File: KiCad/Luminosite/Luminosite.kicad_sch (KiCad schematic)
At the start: 1 part, among them U4 ESP32-C3_SUPERMINI_TH

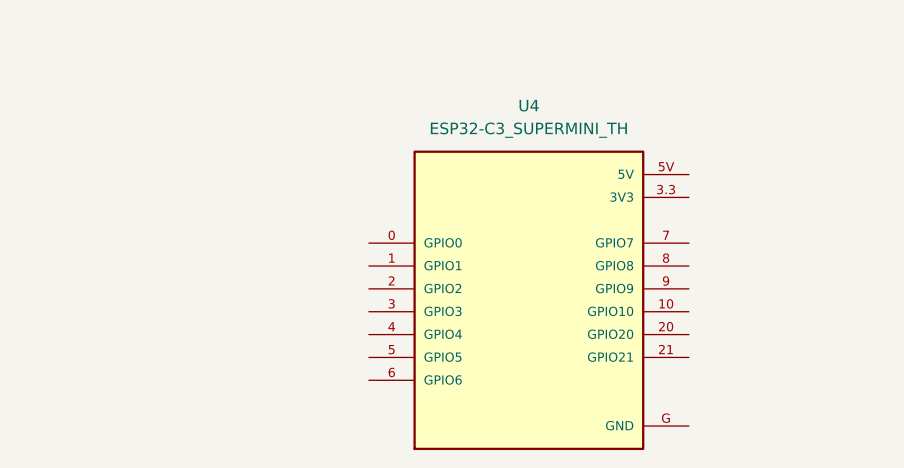
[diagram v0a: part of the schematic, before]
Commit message: Commencement du PCB
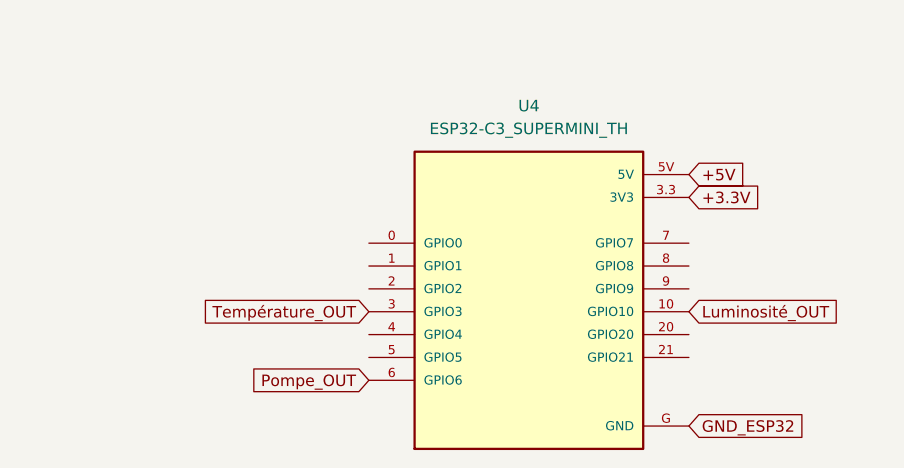
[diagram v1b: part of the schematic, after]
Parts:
- U4: footprint ESP32-C3_SUPERMINI_TH:MODULE_ESP32-C3_SUPERMINI_TH -> ESP32-C3-Supermini:MODULE_ESP32-C3_SUPERMINI_TH
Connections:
- net Luminosité_OUT: now reaches U4.10 (GPIO10)
- net Température_OUT: now reaches U4.3 (GPIO3)
- net +3.3V: now reaches U4.3.3 (3V3)
- net +5V: now reaches U4.5V
- net Pompe_OUT: now reaches U4.6 (GPIO6)
- net GND_ESP32: now reaches U4.G (GND)
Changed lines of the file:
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@@
 	(generator_version "10.0")
 	(paper "A4")
+	(global_label "Température_OUT"
+		(shape input)
+		(at 104.14 116.84 180)
+		(fields_autoplaced yes)
+		(effects
+			(font
+				(size 1.27 1.27)
+			)
+			(justify right)
+		)
+		(property "Intersheetrefs" "${INTERSHEET_REFS}"
+			(at 85.541 116.84 0)
+			(hide yes)
+			(show_name no)
+			(do_not_autoplace no)
+			(effects
+				(font
+					(size 1.27 1.27)
+				)
+				(justify right)
+			)
+		)
+	)
+	(global_label "Pompe_OUT"
+		(shape input)
+		(at 104.14 124.46 180)
+		(fields_autoplaced yes)
+		(effects
+			(font
+				(size 1.27 1.27)
+			)
+			(justify right)
+		)
+		(property "Intersheetrefs" "${INTERSHEET_REFS}"
+			(at 90.8629 124.46 0)
+			(hide yes)
+			(show_name no)
+			(do_not_autoplace no)
+			(effects
+				(font
+					(size 1.27 1.27)
+				)
+				(justify right)
+			)
+		)
+	)
+	(global_label "+3.3V"
+		(shape input)
+		(at 139.7 104.14 0)
+		(fields_autoplaced yes)
+		(effects
+			(font
+				(size 1.27 1.27)
+			)
+			(justify left)
+		)
+		(property "Intersheetrefs" "${INTERSHEET_REFS}"
+			(at 148.37 104.14 0)
+			(hide yes)
+			(show_name no)
+			(do_not_autoplace no)
+			(effects
+				(font
+					(size 1.27 1.27)
+				)
+				(justify left)
+			)
+		)
+	)
+	(global_label "GND_ESP32"
+		(shape input)
+		(at 139.7 129.54 0)
+		(fields_autoplaced yes)
+		(effects
+			(font
+				(size 1.27 1.27)
+			)
+			(justify left)
+		)
+		(property "Intersheetrefs" "${INTERSHEET_REFS}"
+			(at 152.9166 129.54 0)
+			(hide yes)
+			(show_name no)
+			(do_not_autoplace no)
+			(effects
+				(font
+					(size 1.27 1.27)
+				)
+				(justify left)
+			)
+		)
+	)
+	(global_label "+5V"
+		(shape input)
+		(at 139.7 101.6 0)
+		(fields_autoplaced yes)
+		(effects
+			(font
+				(size 1.27 1.27)
+			)
+			(justify left)
+		)
+		(property "Intersheetrefs" "${INTERSHEET_REFS}"
+			(at 145.9015 101.6 0)
+			(hide yes)
+			(show_name no)
+			(do_not_autoplace no)
+			(effects
+				(font
+					(size 1.27 1.27)
+				)
+				(justify left)
+			)
+		)
+	)
+	(global_label "Luminosité_OUT"
+		(shape input)
+		(at 139.7 116.84 0)
+		(fields_autoplaced yes)
+		(effects
+			(font
+				(size 1.27 1.27)
+			)
+			(justify left)
+		)
+		(property "Intersheetrefs" "${INTERSHEET_REFS}"
+			(at 156.8476 116.84 0)
+			(hide yes)
+			(show_name no)
+			(do_not_autoplace no)
+			(effects
+				(font
+					(size 1.27 1.27)
+				)
+				(justify left)
+			)
+		)
+	)
 	(symbol
 		(lib_id "ESP32-C3-Supermini:ESP32-C3_SUPERMINI_TH")
 		(at 121.92 114.3 0)
 		(unit 1)
+		(body_style 1)
 		(exclude_from_sim no)
 		(in_bom yes)
 		(on_board yes)
+		(in_pos_files yes)
 		(dnp no)
 		(fields_autoplaced yes)
 		(property "Reference" "U4"
 			(at 121.92 93.98 0)
+			(show_name no)
+			(do_not_autoplace no)
 			(effects
 				(font
@@
 		(property "Value" "ESP32-C3_SUPERMINI_TH"
 			(at 121.92 96.52 0)
-			(effects
-				(font
-					(size 1.27 1.27)
-				)
-			)
-		)
-		(property "Footprint" "ESP32-C3_SUPERMINI_TH:MODULE_ESP32-C3_SUPERMINI_TH"
-			(at 121.92 114.3 0)
-			(effects
-				(font
-					(size 1.27 1.27)
-				)
-				(justify bottom)
-				(hide yes)
+			(show_name no)
+			(do_not_autoplace no)
+			(effects
+				(font
+					(size 1.27 1.27)
+				)
+			)
+		)
+		(property "Footprint" "ESP32-C3-Supermini:MODULE_ESP32-C3_SUPERMINI_TH"
+			(at 121.92 114.3 0)
+			(hide yes)
+			(show_name no)
+			(do_not_autoplace no)
+			(effects
+				(font
+					(size 1.27 1.27)
+				)
+				(justify bottom)
 			)
 		)
 		(property "Datasheet" ""
 			(at 121.92 114.3 0)
-			(effects
-				(font
-					(size 1.27 1.27)
-				)
-				(hide yes)
+			(hide yes)
+			(show_name no)
+			(do_not_autoplace no)
+			(effects
+				(font
+					(size 1.27 1.27)
+				)
 			)
 		)
 		(property "Description" ""
 			(at 121.92 114.3 0)
-			(effects
-				(font
-					(size 1.27 1.27)
-				)
-				(hide yes)
+			(hide yes)
+			(show_name no)
+			(do_not_autoplace no)
+			(effects
+				(font
+					(size 1.27 1.27)
+				)
 			)
 		)
 		(property "MF" "Espressif Systems"
 			(at 121.92 114.3 0)
-			(effects
-				(font
-					(size 1.27 1.27)
-				)
-				(justify bottom)
-				(hide yes)
+			(hide yes)
+			(show_name no)
+			(do_not_autoplace no)
+			(effects
+				(font
+					(size 1.27 1.27)
+				)
+				(justify bottom)
 			)
 		)
 		(property "Description_1" "Super tiny ESP32-C3 board"
 			(at 121.92 114.3 0)
-			(effects
-				(font
-					(size 1.27 1.27)
-				)
-				(justify bottom)
-				(hide yes)
+			(hide yes)
+			(show_name no)
+			(do_not_autoplace no)
+			(effects
+				(font
+					(size 1.27 1.27)
+				)
+				(justify bottom)
 			)
 		)
 		(property "CREATOR" "DIZAR"
 			(at 121.92 114.3 0)
-			(effects
-				(font
-					(size 1.27 1.27)
-				)
-				(justify bottom)
-				(hide yes)
+			(hide yes)
+			(show_name no)
+			(do_not_autoplace no)
+			(effects
+				(font
+					(size 1.27 1.27)
+				)
+				(justify bottom)
 			)
 		)
 		(property "Price" "None"
 			(at 121.92 114.3 0)
-			(effects
-				(font
-					(size 1.27 1.27)
-				)
-				(justify bottom)
-				(hide yes)
+			(hide yes)
+			(show_name no)
+			(do_not_autoplace no)
+			(effects
+				(font
+					(size 1.27 1.27)
+				)
+				(justify bottom)
 			)
 		)
 		(property "Package" "Package"
 			(at 121.92 114.3 0)
-			(effects
-				(font
-					(size 1.27 1.27)
-				)
-				(justify bottom)
-				(hide yes)
+			(hide yes)
+			(show_name no)
+			(do_not_autoplace no)
+			(effects
+				(font
+					(size 1.27 1.27)
+				)
+				(justify bottom)
 			)
 		)
 		(property "Check_prices" "https://www.snapeda.com/parts/ESP32-C3%20SuperMini_TH/Espressif+Systems/view-part/?ref=eda"
 			(at 121.92 114.3 0)
-			(effects
-				(font
-					(size 1.27 1.27)
-				)
-				(justify bottom)
-				(hide yes)
+			(hide yes)
+			(show_name no)
+			(do_not_autoplace no)
+			(effects
+				(font
+					(size 1.27 1.27)
+				)
+				(justify bottom)
 			)
 		)
 		(property "STANDARD" "IPC-7351B"
 			(at 121.92 114.3 0)
-			(effects
-				(font
-					(size 1.27 1.27)
-				)
-				(justify bottom)
-				(hide yes)
+			(hide yes)
+			(show_name no)
+			(do_not_autoplace no)
+			(effects
+				(font
+					(size 1.27 1.27)
+				)
+				(justify bottom)
 			)
 		)
 		(property "VERIFIER" ""
 			(at 121.92 114.3 0)
-			(effects
-				(font
-					(size 1.27 1.27)
-				)
-				(justify bottom)
-				(hide yes)
+			(hide yes)
+			(show_name no)
+			(do_not_autoplace no)
+			(effects
+				(font
+					(size 1.27 1.27)
+				)
+				(justify bottom)
 			)
 		)
 		(property "SnapEDA_Link" "https://www.snapeda.com/parts/ESP32-C3%20SuperMini_TH/Espressif+Systems/view-part/?ref=snap"
 			(at 121.92 114.3 0)
-			(effects
-				(font
-					(size 1.27 1.27)
-				)
-				(justify bottom)
-				(hide yes)
+			(hide yes)
+			(show_name no)
+			(do_not_autoplace no)
+			(effects
+				(font
+					(size 1.27 1.27)
+				)
+				(justify bottom)
 			)
 		)
 		(property "MP" "ESP32-C3 SuperMini_TH"
 			(at 121.92 114.3 0)
-			(effects
-				(font
-					(size 1.27 1.27)
-				)
-				(justify bottom)
-				(hide yes)
+			(hide yes)
+			(show_name no)
+			(do_not_autoplace no)
+			(effects
+				(font
+					(size 1.27 1.27)
+				)
+				(justify bottom)
 			)
 		)
 		(property "Availability" "Not in stock"
 			(at 121.92 114.3 0)
-			(effects
-				(font
-					(size 1.27 1.27)
-				)
-				(justify bottom)
-				(hide yes)
+			(hide yes)
+			(show_name no)
+			(do_not_autoplace no)
+			(effects
+				(font
+					(size 1.27 1.27)
+				)
+				(justify bottom)
 			)
 		)
 		(property "MANUFACTURER" "Espressif Systems"
 			(at 121.92 114.3 0)
-			(effects
-				(font
-					(size 1.27 1.27)
-				)
-				(justify bottom)
-				(hide yes)
+			(hide yes)
+			(show_name no)
+			(do_not_autoplace no)
+			(effects
+				(font
+					(size 1.27 1.27)
+				)
+				(justify bottom)
 			)
 		)
@@
 		)
 		(fill
-			(color 0 0 0 0.0000)
+			(color 0 0 0 0)
 		)
 		(property "Sheetname" "Pompe"
 			(at 105.41 14.5284 0)
+			(show_name no)
+			(do_not_autoplace no)
 			(effects
 				(font
@@
 		(property "Sheetfile" "Pompe.kicad_sch"
 			(at 105.41 52.6546 0)
+			(show_name no)
+			(do_not_autoplace no)
 			(effects
 				(font
@@
 		(property "Field2" ""
 			(at 105.41 15.24 0)
-			(effects
-				(font
+			(show_name no)
+			(do_not_autoplace no)
+			(effects
+				(font
